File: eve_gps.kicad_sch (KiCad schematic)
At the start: 9 parts, among them J14 BMI-S-101, J15 GNSS SMA

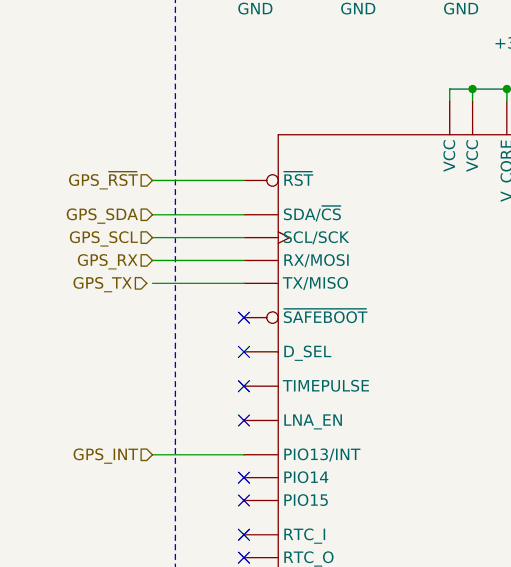
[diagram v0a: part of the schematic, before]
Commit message: addressed PR comments
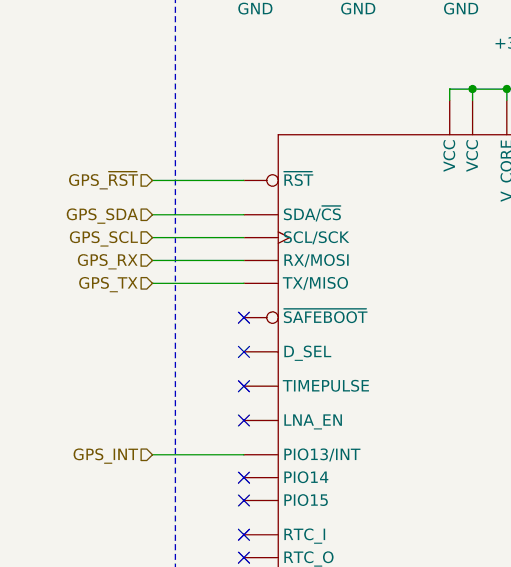
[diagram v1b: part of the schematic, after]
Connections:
- net GPS_TX: now also U39.J5 (TX/MISO)
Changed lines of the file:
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@@
 	(hierarchical_label "GPS_TX"
 		(shape input)
-		(at 78.105 97.79 180)
+		(at 78.74 97.79 180)
 		(fields_autoplaced yes)
 		(effects
@@
 		(on_board yes)
 		(dnp no)
-		(property "Reference" "#PWR0193"
+		(property "Reference" "#PWR0194"
 			(at 194.31 97.79 0)
 			(effects
@@
 			(project "rocket2-ecu"
 				(path "/02606b2c-b376-4ffb-9781-f9cea3f70994/33703977-e0e9-46ee-bac6-f4661129caa1"
-					(reference "#PWR0193")
+					(reference "#PWR0194")
 					(unit 1)
 				)
@@
 		(on_board yes)
 		(dnp no)
-		(property "Reference" "#PWR0184"
+		(property "Reference" "#PWR0185"
 			(at 119.38 78.74 0)
 			(effects
@@
 			(project "rocket2-ecu"
 				(path "/02606b2c-b376-4ffb-9781-f9cea3f70994/33703977-e0e9-46ee-bac6-f4661129caa1"
-					(reference "#PWR0184")
+					(reference "#PWR0185")
 					(unit 1)
 				)
@@
 		(on_board yes)
 		(dnp no)
-		(property "Reference" "#PWR0182"
+		(property "Reference" "#PWR0183"
 			(at 113.03 62.23 0)
 			(effects
@@
 			(project "rocket2-ecu"
 				(path "/02606b2c-b376-4ffb-9781-f9cea3f70994/33703977-e0e9-46ee-bac6-f4661129caa1"
-					(reference "#PWR0182")
+					(reference "#PWR0183")
 					(unit 1)
 				)
@@
 		(on_board yes)
 		(dnp no)
-		(property "Reference" "#PWR0191"
+		(property "Reference" "#PWR0192"
 			(at 147.32 69.85 0)
 			(effects
@@
 			(project "rocket2-ecu"
 				(path "/02606b2c-b376-4ffb-9781-f9cea3f70994/33703977-e0e9-46ee-bac6-f4661129caa1"
-					(reference "#PWR0191")
+					(reference "#PWR0192")
 					(unit 1)
 				)
@@
 		(on_board yes)
 		(dnp no)
-		(property "Reference" "#PWR0179"
+		(property "Reference" "#PWR0180"
 			(at 90.17 69.85 0)
 			(effects
@@
 			(project "rocket2-ecu"
 				(path "/02606b2c-b376-4ffb-9781-f9cea3f70994/33703977-e0e9-46ee-bac6-f4661129caa1"
-					(reference "#PWR0179")
+					(reference "#PWR0180")
 					(unit 1)
 				)
@@
 		(on_board yes)
 		(dnp no)
-		(property "Reference" "#PWR0186"
+		(property "Reference" "#PWR0187"
 			(at 124.46 62.23 0)
 			(effects
@@
 			(project "rocket2-ecu"
 				(path "/02606b2c-b376-4ffb-9781-f9cea3f70994/33703977-e0e9-46ee-bac6-f4661129caa1"
-					(reference "#PWR0186")
+					(reference "#PWR0187")
 					(unit 1)
 				)
@@
 		(on_board yes)
 		(dnp no)
-		(property "Reference" "#PWR0189"
+		(property "Reference" "#PWR0190"
 			(at 135.89 69.85 0)
 			(effects
@@
 			(project "rocket2-ecu"
 				(path "/02606b2c-b376-4ffb-9781-f9cea3f70994/33703977-e0e9-46ee-bac6-f4661129caa1"
-					(reference "#PWR0189")
+					(reference "#PWR0190")
 					(unit 1)
 				)
@@
 		(on_board yes)
 		(dnp no)
-		(property "Reference" "#PWR0180"
+		(property "Reference" "#PWR0181"
 			(at 101.6 62.23 0)
 			(effects
@@
 			(project "rocket2-ecu"
 				(path "/02606b2c-b376-4ffb-9781-f9cea3f70994/33703977-e0e9-46ee-bac6-f4661129caa1"
-					(reference "#PWR0180")
+					(reference "#PWR0181")
 					(unit 1)
 				)
@@
 		(on_board yes)
 		(dnp no)
-		(property "Reference" "#PWR0183"
+		(property "Reference" "#PWR0184"
 			(at 113.03 69.85 0)
 			(effects
@@
 			(project "rocket2-ecu"
 				(path "/02606b2c-b376-4ffb-9781-f9cea3f70994/33703977-e0e9-46ee-bac6-f4661129caa1"
-					(reference "#PWR0183")
+					(reference "#PWR0184")
 					(unit 1)
 				)
@@
 		(on_board yes)
 		(dnp no)
-		(property "Reference" "#PWR0190"
+		(property "Reference" "#PWR0191"
 			(at 147.32 62.23 0)
 			(effects
@@
 			(project "rocket2-ecu"
 				(path "/02606b2c-b376-4ffb-9781-f9cea3f70994/33703977-e0e9-46ee-bac6-f4661129caa1"
-					(reference "#PWR0190")
+					(reference "#PWR0191")
 					(unit 1)
 				)
@@
 		(on_board yes)
 		(dnp no)
-		(property "Reference" "#PWR0192"
+		(property "Reference" "#PWR0193"
 			(at 168.91 151.13 0)
 			(effects
@@
 			(project "rocket2-ecu"
 				(path "/02606b2c-b376-4ffb-9781-f9cea3f70994/33703977-e0e9-46ee-bac6-f4661129caa1"
-					(reference "#PWR0192")
+					(reference "#PWR0193")
 					(unit 1)
 				)
@@
 		(on_board yes)
 		(dnp no)
-		(property "Reference" "#PWR0185"
+		(property "Reference" "#PWR0186"
 			(at 119.38 147.32 0)
 			(effects
@@
 			(project "rocket2-ecu"
 				(path "/02606b2c-b376-4ffb-9781-f9cea3f70994/33703977-e0e9-46ee-bac6-f4661129caa1"
-					(reference "#PWR0185")
+					(reference "#PWR0186")
 					(unit 1)
 				)
@@
 		(on_board yes)
 		(dnp no)
-		(property "Reference" "#PWR0187"
+		(property "Reference" "#PWR0188"
 			(at 124.46 69.85 0)
 			(effects
@@
 			(project "rocket2-ecu"
 				(path "/02606b2c-b376-4ffb-9781-f9cea3f70994/33703977-e0e9-46ee-bac6-f4661129caa1"
-					(reference "#PWR0187")
+					(reference "#PWR0188")
 					(unit 1)
 				)
@@
 		(on_board yes)
 		(dnp no)
-		(property "Reference" "#PWR0178"
+		(property "Reference" "#PWR0179"
 			(at 90.17 62.23 0)
 			(effects
@@
 			(project "rocket2-ecu"
 				(path "/02606b2c-b376-4ffb-9781-f9cea3f70994/33703977-e0e9-46ee-bac6-f4661129caa1"
-					(reference "#PWR0178")
+					(reference "#PWR0179")
 					(unit 1)
 				)
@@
 		(on_board yes)
 		(dnp no)
-		(property "Reference" "#PWR0181"
+		(property "Reference" "#PWR0182"
 			(at 101.6 69.85 0)
 			(effects
@@
 			(project "rocket2-ecu"
 				(path "/02606b2c-b376-4ffb-9781-f9cea3f70994/33703977-e0e9-46ee-bac6-f4661129caa1"
-					(reference "#PWR0181")
+					(reference "#PWR0182")
 					(unit 1)
 				)
@@
 		(on_board yes)
 		(dnp no)
-		(property "Reference" "#PWR0188"
+		(property "Reference" "#PWR0189"
 			(at 135.89 62.23 0)
 			(effects
@@
 			(project "rocket2-ecu"
 				(path "/02606b2c-b376-4ffb-9781-f9cea3f70994/33703977-e0e9-46ee-bac6-f4661129caa1"
-					(reference "#PWR0188")
-					(unit 1)
-				)
+					(reference "#PWR0189")
+					(unit 1)
+				)
